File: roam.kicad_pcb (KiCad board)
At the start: 4 copper layers, 100 x 60 mm, 302 parts, among them IC2 MCP73833T-FCI/MF, J1 SIM8060-6-0-14-00-A, J2 Battery, J3 Conn_01x03_Pin, J4 USB_B_Micro, J5 Conn_01x03_Pin, Q3 MMBT3904, Q4 MMBT3904, Q5 BC846A,215, Q6 BC846A,215, Q7 BC846A,215, U1 NUP4202, U10 LTV-217, U11 W25N512GVEIG, U12 LM3671MF-3.3/NOPB, U13 LIS2DH12TR, U14 MAX17643ATC+, U15 FDMC86139P, U16 MCP2562-E/MF, U17 LTV-217, U18 MP3423GG, U19 MX25R6435FZNIL0, U2 MDBT50Q-1M, U20 TPS566242DRLR, U22 MAX13487EESAT, U23 TXS0102DCU, U24 LP5907MFX-3.3, U27 EG915ULAAB-N05-SNNSA, U28 LC29H, U29 USBLC6-2SC6, U31 B8389, U32 LP5907MFX-3.3, U4 STM32F105RBT6, U5 TXB0108DQSR, U6 MCP2562-E/MF, U7 LM66100DCKR, U8 GP.1575.25.2.A.02, U9 LM66100DCKR, Y1 25MHz

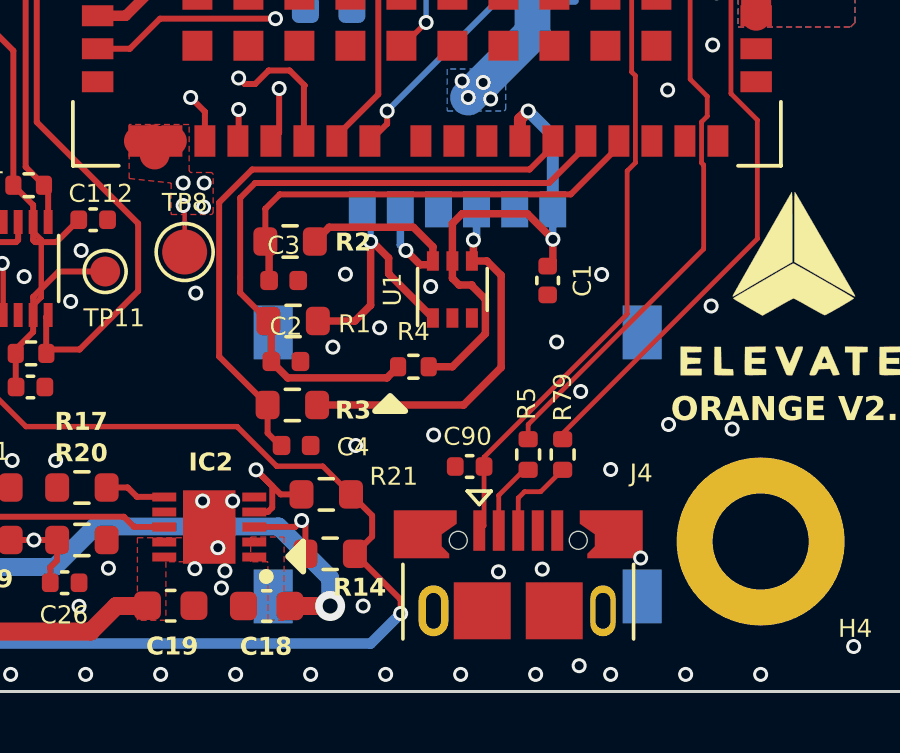
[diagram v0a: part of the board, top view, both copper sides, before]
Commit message: saved
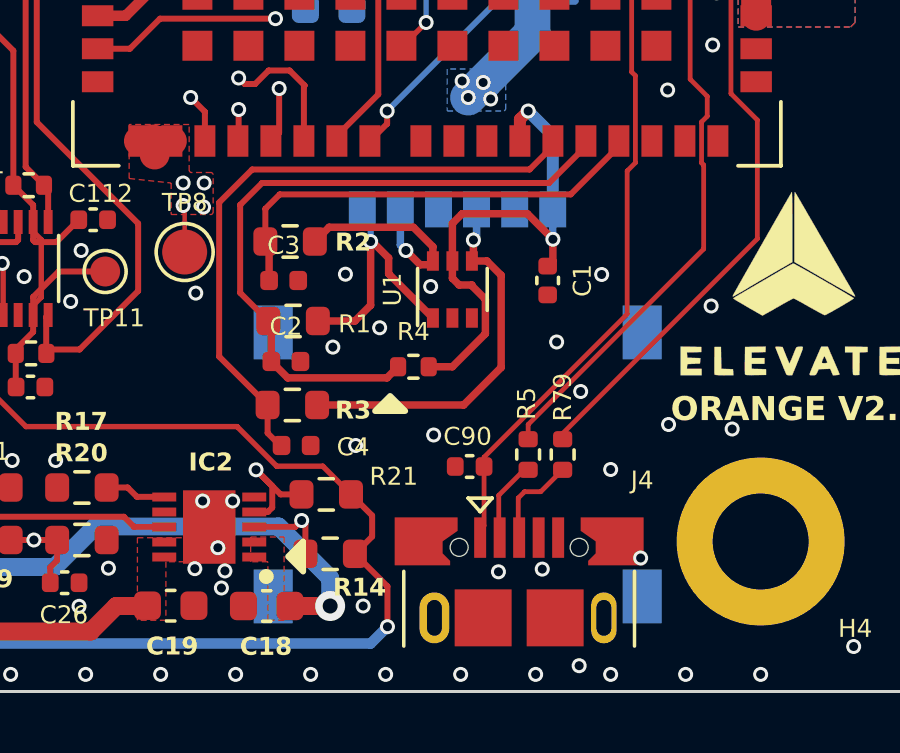
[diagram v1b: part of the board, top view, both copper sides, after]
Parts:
- moved J4 0.24 mm to (172.9, 142.2)
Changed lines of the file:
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@@
     (pad_to_mask_clearance 0)
     (aux_axis_origin 100 145)
-    (grid_origin 144.7 125.95)
+    (grid_origin 176.91 126.66)
     (pcbplotparams
       (layerselection 0x000d0fc_ffffffff)
@@
   )
   (footprint "Connector_USB:USB_Micro-B_XKB_U254-051T-4BH83-F1S" (layer "F.Cu")
-    (at 172.92 141.92)
+    (at 172.95 142.155)
     (descr "XKB Connectivity, USB Micro-B, right-angle, SMT, https://datasheet.lcsc.com/lcsc/2206091745_XKB-Connectivity-U254-051T-4BH83-F1S_C397452.pdf")
     (tags "USB Micro-B Receptacle SMD")
@@
   (segment (start 133.57 91.075) (end 133.57 92.91234) (width 0.2) (layer "B.Cu") (net 18))
   (segment (start 164.69 134) (end 165.235 134.545) (width 0.25) (layer "F.Cu") (net 19))
-  (segment (start 163.65 128.55) (end 163.65 131.2) (width 0.2) (layer "F.Cu") (net 19))
-  (segment (start 163.65 131.2) (end 163.65 131.71) (width 0.2) (layer "F.Cu") (net 19))
+  (segment (start 175.175 126.65) (end 175.175 126.825) (width 0.2) (layer "F.Cu") (net 19))
+  (segment (start 164.38 128.05) (end 163.65 128.78) (width 0.2) (layer "F.Cu") (net 19))
+  (segment (start 163.65 128.78) (end 163.65 131.71) (width 0.2) (layer "F.Cu") (net 19))
   (segment (start 165.235 134.545) (end 168.545 134.545) (width 0.25) (layer "F.Cu") (net 19))
-  (segment (start 175.175 126.825) (end 173.95 128.05) (width 0.2) (layer "F.Cu") (net 19))
-  (segment (start 173.95 128.05) (end 164.15 128.05) (width 0.2) (layer "F.Cu") (net 19))
+  (segment (start 163.65 131.71) (end 164.59 132.65) (width 0.2) (layer "F.Cu") (net 19))
   (segment (start 164.69 134) (end 164.69 132.75) (width 0.25) (layer "F.Cu") (net 19))
   (segment (start 168.545 134.545) (end 168.915 134.175) (width 0.25) (layer "F.Cu") (net 19))
-  (segment (start 175.175 126.65) (end 175.175 126.825) (width 0.2) (layer "F.Cu") (net 19))
+  (segment (start 175.175 126.825) (end 173.95 128.05) (width 0.2) (layer "F.Cu") (net 19))
+  (segment (start 173.95 128.05) (end 164.38 128.05) (width 0.2) (layer "F.Cu") (net 19))
   (segment (start 164.69 132.75) (end 164.59 132.65) (width 0.25) (layer "F.Cu") (net 19))
-  (segment (start 163.65 131.71) (end 164.59 132.65) (width 0.2) (layer "F.Cu") (net 19))
-  (segment (start 164.15 128.05) (end 163.65 128.55) (width 0.2) (layer "F.Cu") (net 19))
   (segment (start 176.275 126.65) (end 176.275 126.825) (width 0.2) (layer "F.Cu") (net 20))
   (segment (start 164.615 130.125) (end 164.49 130) (width 0.25) (layer "F.Cu") (net 20))
@@
   (segment (start 179.55 98.05) (end 180.77 98.05) (width 0.25) (layer "F.Cu") (net 64))
   (segment (start 139.72 88.27) (end 139.72 89.665) (width 0.25) (layer "F.Cu") (net 64))
+  (segment (start 168.56 142.84) (end 168.56 141.495) (width 0.2) (layer "F.Cu") (net 64))
   (segment (start 124 109.02) (end 123.03 109.99) (width 0.25) (layer "F.Cu") (net 64))
   (segment (start 174.775 97.5) (end 174.775 96.625) (width 0.35) (layer "F.Cu") (net 64))
@@
   (segment (start 161.45 101.32) (end 161.9925 101.32) (width 0.35) (layer "F.Cu") (net 64))
   (segment (start 125.05 97.76) (end 125.46 97.76) (width 0.25) (layer "F.Cu") (net 64))
-  (segment (start 169 141.935) (end 167.475 140.41) (width 0.2) (layer "F.Cu") (net 64))
   (segment (start 113.25 100.64) (end 112 100.64) (width 0.2) (layer "F.Cu") (net 64))
   (segment (start 118.9 119.3875) (end 118.75 119.2375) (width 0.6) (layer "F.Cu") (net 64))
@@
   (segment (start 177.525 92.475) (end 182.21 97.16) (width 0.35) (layer "F.Cu") (net 64))
   (segment (start 156.25 129.95) (end 156.25 129.35) (width 0.2) (layer "F.Cu") (net 64))
-  (segment (start 169 142.4) (end 169 141.935) (width 0.2) (layer "F.Cu") (net 64))
   (segment (start 156.51 136.17) (end 155.04 134.7) (width 0.180086) (layer "F.Cu") (net 64))
   (segment (start 112.78 96.8) (end 112.79 96.79) (width 0.25) (layer "F.Cu") (net 64))
@@
   (segment (start 125.05 97.76) (end 125.05 98.575) (width 0.35) (layer "F.Cu") (net 64))
   (segment (start 119.8 119.3875) (end 118.9 119.3875) (width 0.6) (layer "F.Cu") (net 64))
+  (segment (start 168.56 141.495) (end 167.475 140.41) (width 0.2) (layer "F.Cu") (net 64))
   (segment (start 139.7 88.25) (end 139.72 88.27) (width 0.25) (layer "F.Cu") (net 64))
   (segment (start 126.825 102.4) (end 127.075 102.15) (width 0.35) (layer "F.Cu") (net 64))
@@
   (via (at 115.68 117.3875) (size 0.5) (drill 0.3) (layers "F.Cu" "B.Cu") (net 64))
   (via (at 169.05 91.3) (size 0.5) (drill 0.3) (layers "F.Cu" "B.Cu") (net 64))
-  (via (at 169 142.4) (size 0.5) (drill 0.3) (layers "F.Cu" "B.Cu") (net 64))
+  (via (at 168.56 142.84) (size 0.5) (drill 0.3) (layers "F.Cu" "B.Cu") (net 64))
   (via (at 132.45 104.85) (size 0.5) (drill 0.3) (layers "F.Cu" "B.Cu") (net 64))
   (via (at 139.7 88.25) (size 0.5) (drill 0.3) (layers "F.Cu" "B.Cu") (net 64))
@@
   (segment (start 127.8 98.35) (end 127.8 99.7) (width 0.6) (layer "B.Cu") (net 64))
   (segment (start 126.45 102.394473) (end 126.45 101.05) (width 0.6) (layer "B.Cu") (net 64))
+  (segment (start 123.965 136.765) (end 113.1 125.9) (width 0.35) (layer "B.Cu") (net 64))
   (segment (start 130.654999 105.15) (end 126.9 105.15) (width 0.35) (layer "B.Cu") (net 64))
   (segment (start 128.18 110.18) (end 126.9 108.9) (width 0.25) (layer "B.Cu") (net 64))
@@
   (segment (start 131.775 106.54) (end 131.775 106.270001) (width 0.35) (layer "B.Cu") (net 64))
   (segment (start 123.03 110.85) (end 123.03 110.17) (width 0.35) (layer "B.Cu") (net 64))
-  (segment (start 129.206116 143.4) (end 123.965 138.158884) (width 0.35) (layer "B.Cu") (net 64))
-  (segment (start 169 142.4) (end 168 143.4) (width 0.35) (layer "B.Cu") (net 64))
-  (segment (start 123.965 136.765) (end 113.1 125.9) (width 0.35) (layer "B.Cu") (net 64))
   (segment (start 115.68 117.3875) (end 115.7 117.3675) (width 0.6) (layer "B.Cu") (net 64))
   (segment (start 115.1 114.7) (end 115.1 109.375) (width 0.6) (layer "B.Cu") (net 64))
@@
   (segment (start 123.8 114.9) (end 126.9 111.8) (width 0.6) (layer "B.Cu") (net 64))
   (segment (start 115.7 117.3675) (end 115.7 115.3) (width 0.6) (layer "B.Cu") (net 64))
-  (segment (start 168 143.4) (end 129.206116 143.4) (width 0.35) (layer "B.Cu") (net 64))
   (segment (start 123.59 86.49) (end 150.7 86.49) (width 0.5) (layer "B.Cu") (net 64))
   (segment (start 127.6845 87.7) (end 139.15 87.7) (width 0.4) (layer "B.Cu") (net 64))
@@
   (segment (start 118.75 95.75) (end 117.815 94.815) (width 0.25) (layer "B.Cu") (net 64))
   (segment (start 155.21 91) (end 160.05 91) (width 0.5) (layer "B.Cu") (net 64))
-  (segment (start 123.965 138.158884) (end 123.965 136.765) (width 0.35) (layer "B.Cu") (net 64))
   (segment (start 115.68 117.3875) (end 116.65 117.3875) (width 0.6) (layer "B.Cu") (net 64))
   (segment (start 121 106.4) (end 119.51 106.4) (width 0.2) (layer "B.Cu") (net 64))
   (segment (start 136.1 98.4) (end 134.825 99.675) (width 0.4) (layer "B.Cu") (net 64))
+  (segment (start 129.206116 143.4) (end 123.965 138.158884) (width 0.35) (layer "B.Cu") (net 64))
   (segment (start 160.854828 103.204828) (end 160.1 102.45) (width 0.35) (layer "B.Cu") (net 64))
   (segment (start 126.9 102.844473) (end 126.455527 102.4) (width 0.6) (layer "B.Cu") (net 64))
+  (segment (start 168.56 142.84) (end 168 143.4) (width 0.35) (layer "B.Cu") (net 64))
   (segment (start 117.815 94.815) (end 120.73 91.9) (width 0.5) (layer "B.Cu") (net 64))
   (segment (start 119.61 104.4) (end 119.61 106.3) (width 0.2) (layer "B.Cu") (net 64))
@@
   (segment (start 126.9 104.7) (end 126.9 102.844473) (width 0.6) (layer "B.Cu") (net 64))
   (segment (start 127.8 99.7) (end 126.45 101.05) (width 0.6) (layer "B.Cu") (net 64))
+  (segment (start 123.965 138.158884) (end 123.965 136.765) (width 0.35) (layer "B.Cu") (net 64))
   (segment (start 127.85 98.3) (end 127.75 98.2) (width 0.4) (layer "B.Cu") (net 64))
   (segment (start 132.15 105.15) (end 132.45 104.85) (width 0.35) (layer "B.Cu") (net 64))
@@
   (segment (start 127.75 98.2) (end 127.75 89.174391) (width 0.4) (layer "B.Cu") (net 64))
   (segment (start 139.15 87.7) (end 139.7 88.25) (width 0.4) (layer "B.Cu") (net 64))
+  (segment (start 168 143.4) (end 129.206116 143.4) (width 0.35) (layer "B.Cu") (net 64))
   (segment (start 123.03 108.43) (end 123.03 110.85) (width 0.25) (layer "B.Cu") (net 64))
   (segment (start 123.7805 114.8805) (end 123.8 114.9) (width 0.6) (layer "B.Cu") (net 64))
